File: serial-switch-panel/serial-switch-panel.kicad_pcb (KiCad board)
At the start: 2 copper layers, 59 parts, among them J10 Conn_01x01, J11 Conn_01x01, J12 Conn_01x01, J13 Conn_01x01, J14 Conn_01x01, J15 Conn_01x01, J16 Conn_01x01, J17 Conn_01x01, J18 Conn_01x01, J2 2501551-4, J3 Conn_01x01, J4 Conn_01x01, J5 Conn_01x01, J6 Conn_01x01, J7 Conn_01x01, J8 Conn_01x01, J9 Conn_01x01, U1 74LS166, U2 ISL8488E, U3 74LVC1G08, U4 ISL8488E

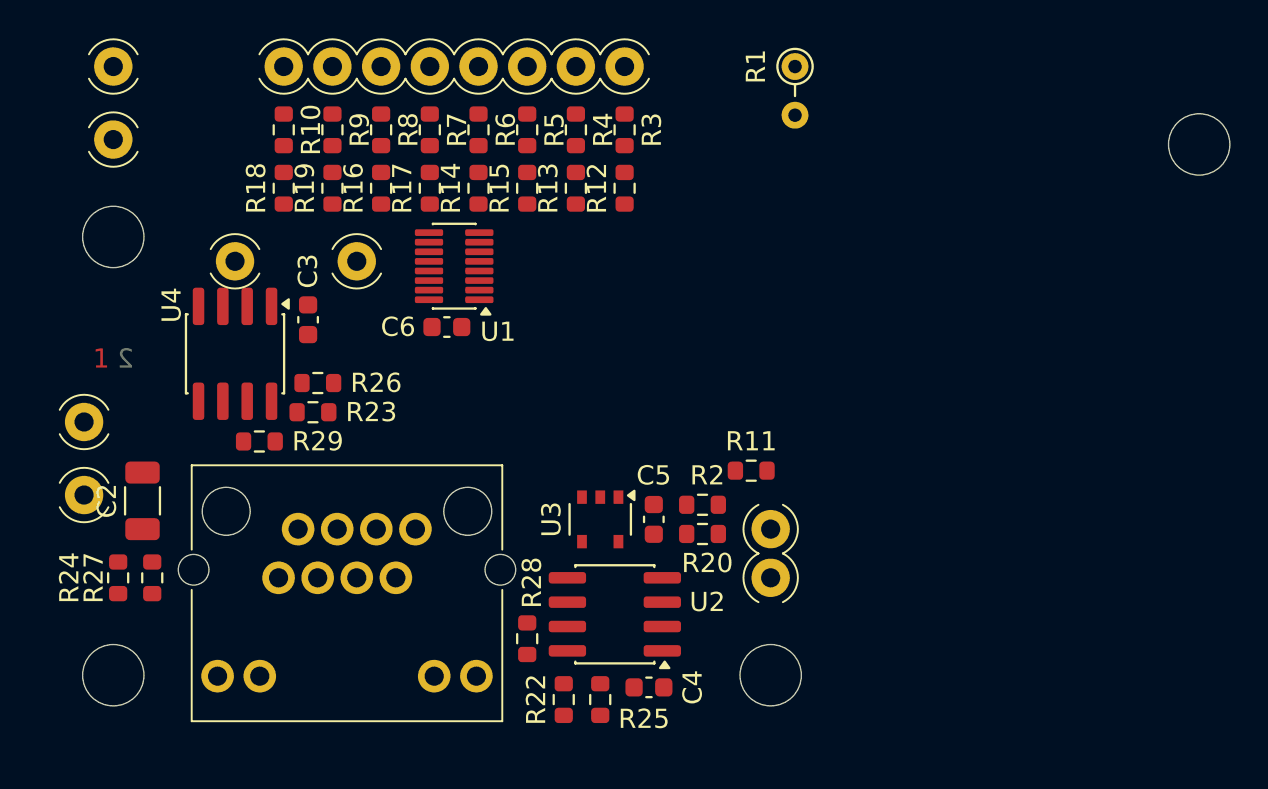
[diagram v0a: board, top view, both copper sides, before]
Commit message: Final? front-panel placement
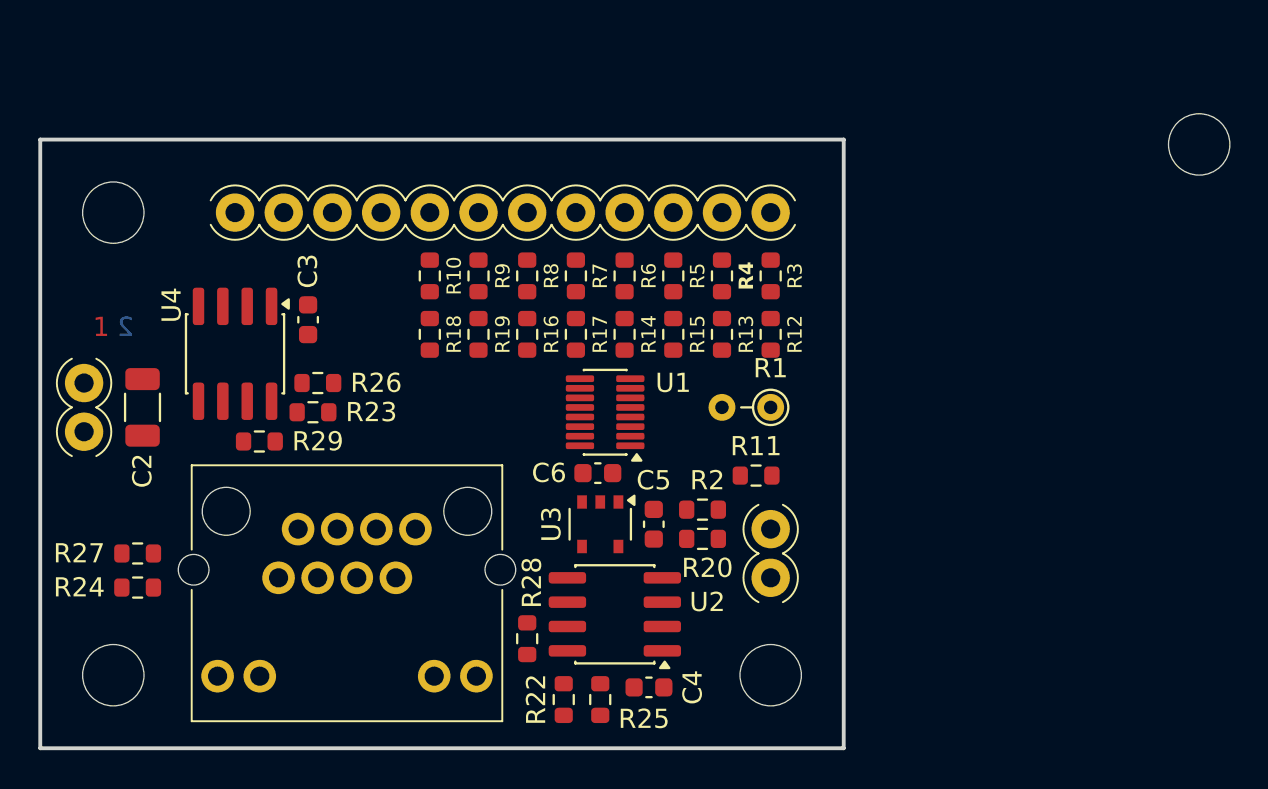
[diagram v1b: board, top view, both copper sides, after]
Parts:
- moved R1 17.8 mm to (138.1, 97.2), turned to 180 degrees
- moved J13 11.7 mm to (112.7, 87.1)
- moved C6 11.0 mm to (129.1, 100.6)
- moved U1 11.0 mm to (129.5, 97.5)
- moved J3 10.8 mm to (138.1, 87.1)
- moved J4 10.8 mm to (135.6, 87.1)
- moved J5 10.8 mm to (133.0, 87.1)
- moved J7 10.8 mm to (127.9, 87.1)
- moved J8 10.8 mm to (125.4, 87.1)
- moved J9 10.8 mm to (122.9, 87.1)
- moved J10 10.8 mm to (120.3, 87.1)
- moved J6 10.8 mm to (130.5, 87.1)
- moved R12 10.8 mm to (138.1, 93.4)
- moved R13 10.8 mm to (135.6, 93.4)
- moved R15 10.8 mm to (133.0, 93.4)
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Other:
- board outline added: 41.9 x 31.8 mm
